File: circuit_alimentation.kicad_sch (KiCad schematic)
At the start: 32 parts, among them U1 STM32-(STM32H745ZIT6)

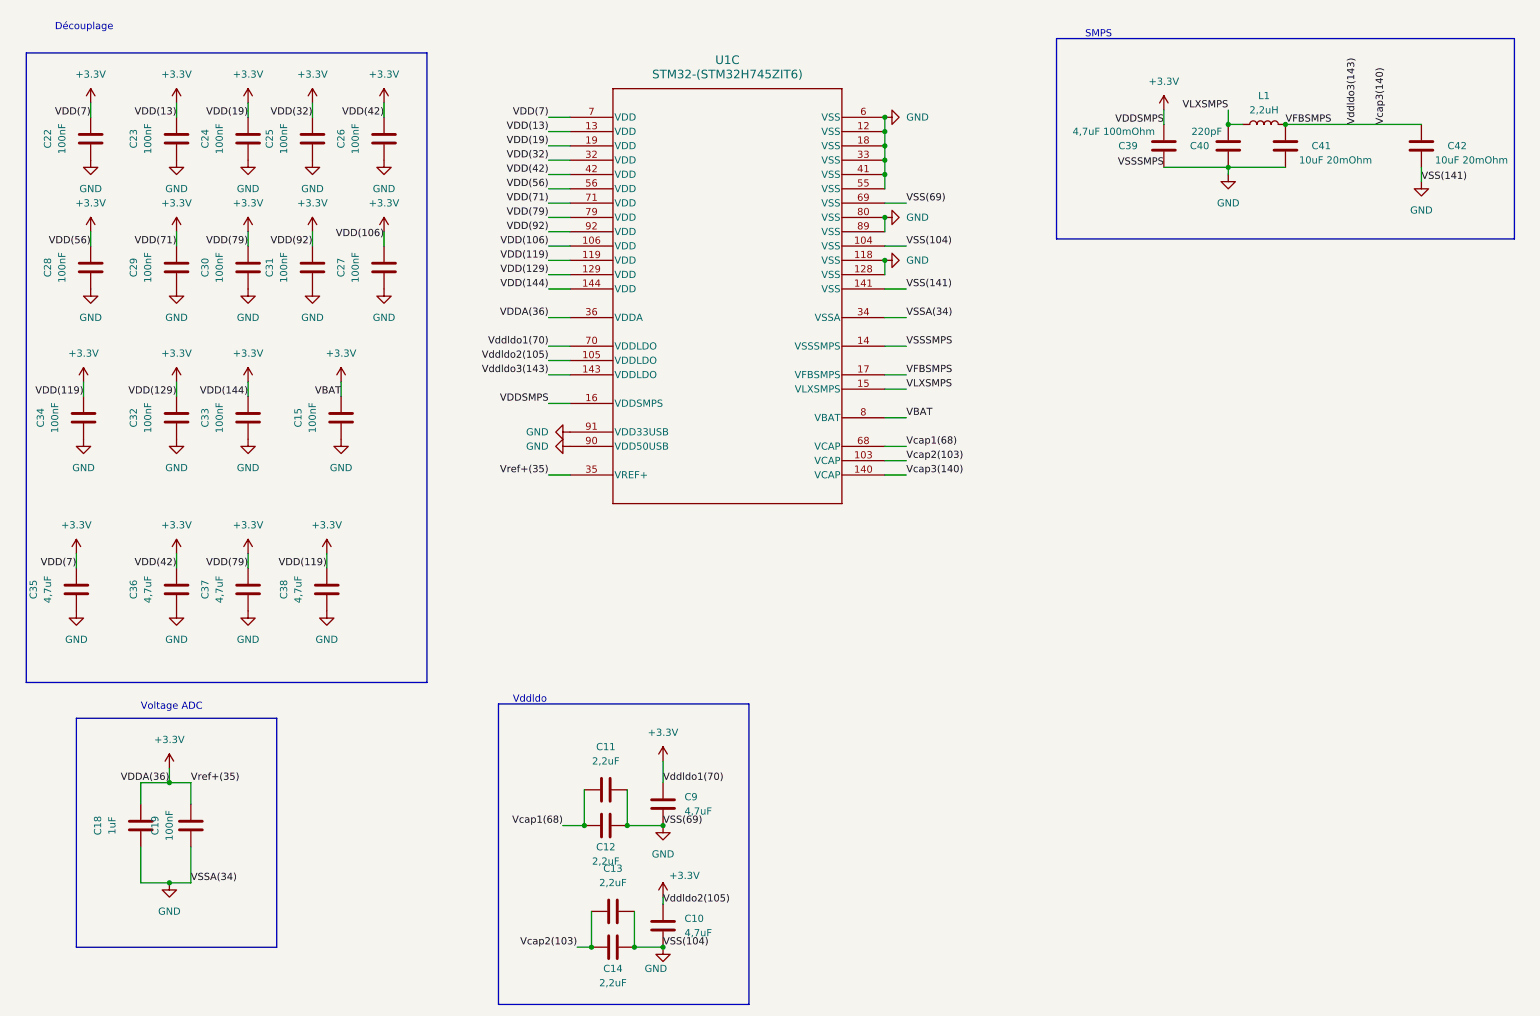
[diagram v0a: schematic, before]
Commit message: ADC_Select
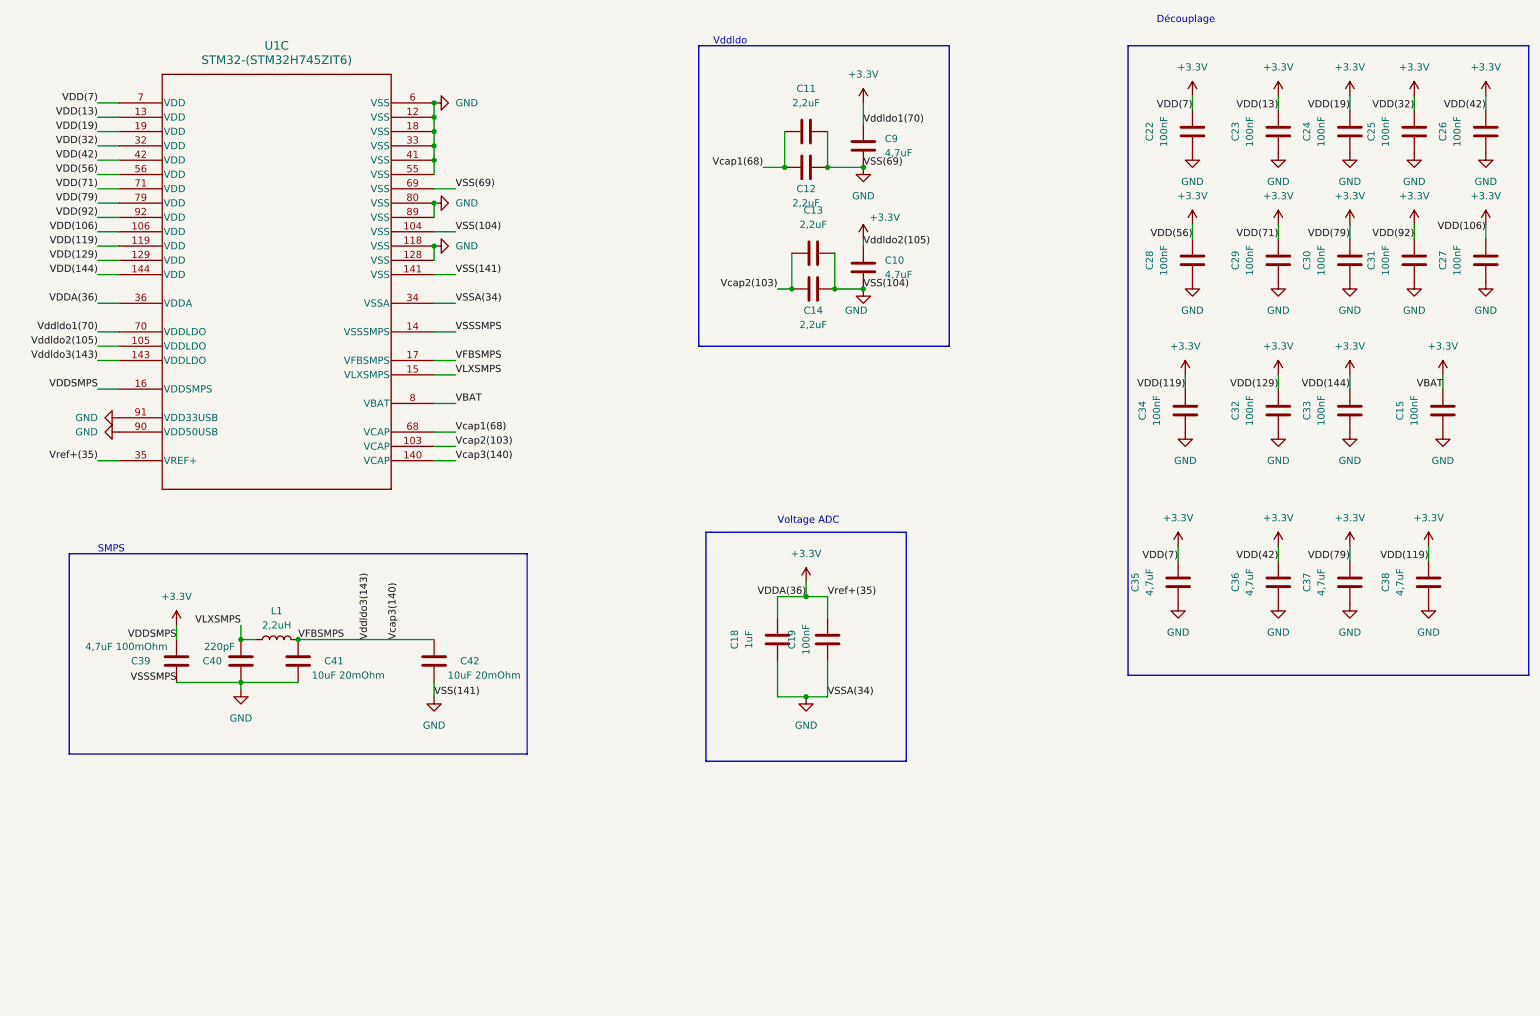
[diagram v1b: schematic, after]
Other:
- moved on the sheet: C10, C11, C12, C13, C14, C15, C18, C19, C22, C23, C24, C25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
